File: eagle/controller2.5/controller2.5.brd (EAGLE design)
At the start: 55.9 x 44.5 mm, 42 parts, among them U1 ATMEGA328P, X1 1501_04

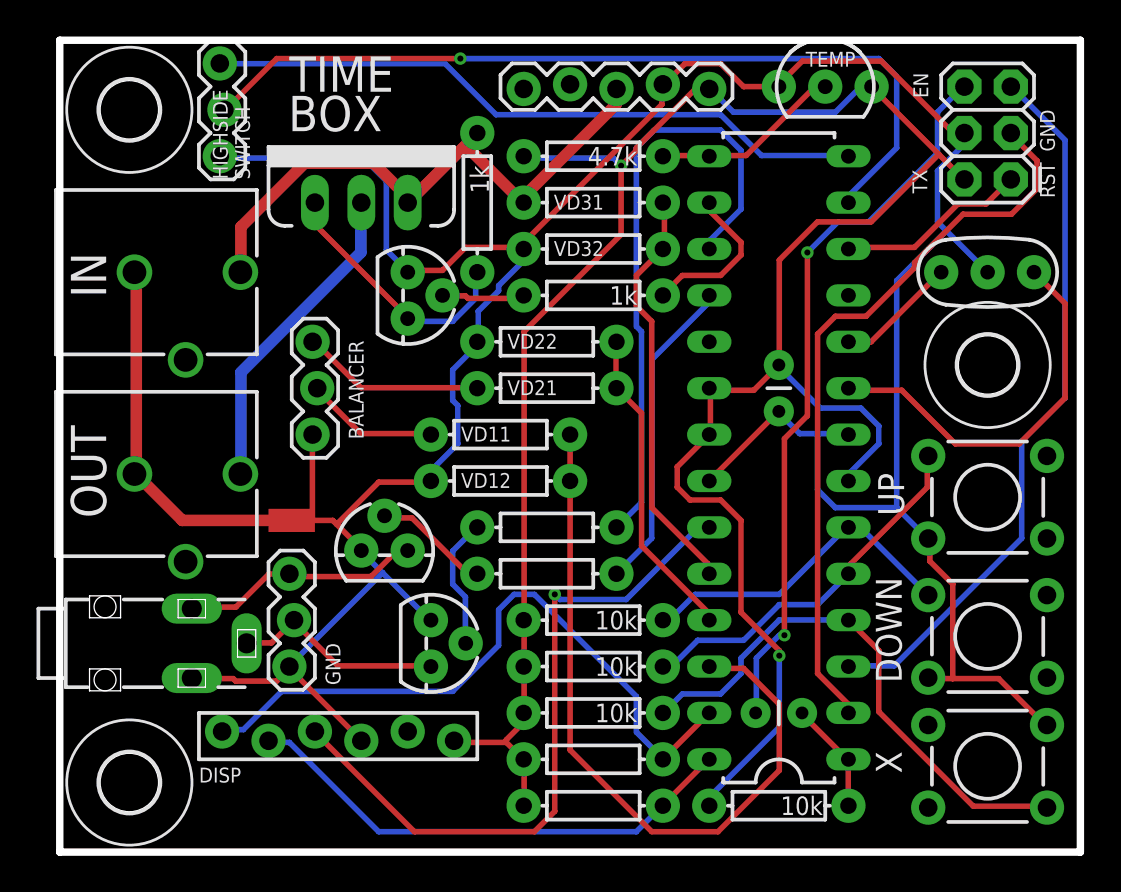
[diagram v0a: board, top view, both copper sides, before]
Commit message: controller2.5: production version
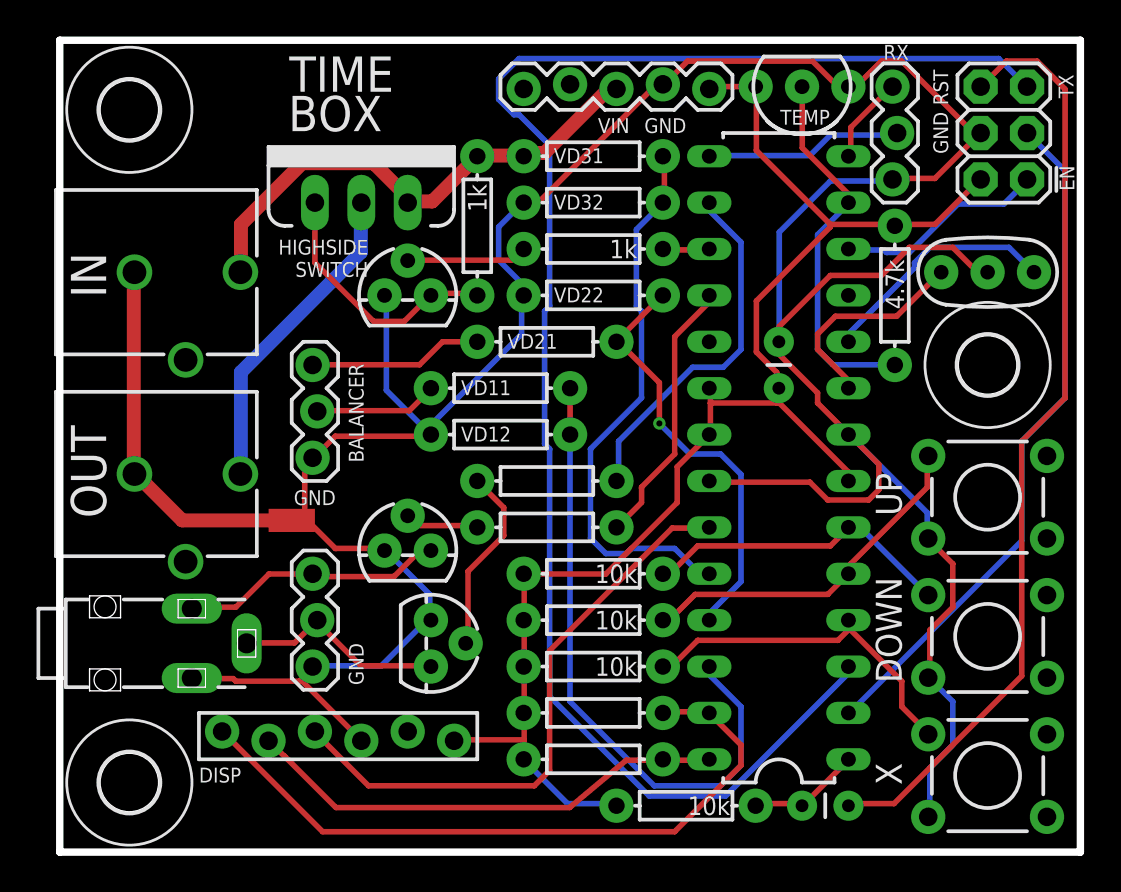
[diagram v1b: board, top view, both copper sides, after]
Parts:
- moved SOFT_SERIAL 36.9 mm to (45.7, 36.8)
- moved RTEMP 18.2 mm to (45.7, 30.5), turned to 90 degrees
- moved C1 7.18 mm to (43.2, 2.54), turned to 180 degrees
- moved R3 5.08 mm to (34.3, 2.54)
- moved C3 3.81 mm to (39.4, 27.9), turned to 270 degrees
- moved VD22 3.59 mm to (29.2, 30.5)
- moved R10 2.54 mm to (29.2, 33.0)
- moved VD21 2.54 mm to (26.7, 27.9)
- moved R7 2.54 mm to (26.7, 17.8)
- moved RB1 2.54 mm to (29.2, 15.2)
- moved R1 2.54 mm to (29.2, 7.62)
- moved R2 2.54 mm to (29.2, 5.08)
- moved RB3 2.54 mm to (29.2, 10.2)
- moved R6 2.54 mm to (26.7, 20.3)
- moved RB2 2.54 mm to (29.2, 12.7)
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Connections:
- removed net DISP_EN: U1.11
- removed net FOO2: U1.19
- net CAM2: now also U1.16; no longer U1.17
- net CAM_EN: now also U1.17; no longer U1.16
- net SOFT_TX: now also U1.15; no longer U1.13
- net TEMP: now also U1.13; no longer U1.15
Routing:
- net VCC: track 130.9 -> 80.8 mm, vias 2 -> 0
- net TX: track 39.3 -> 87.2 mm
- net SOFT_TX: track 46.4 -> 10.9 mm, vias 1 -> 0
- net SOFT_RX: track 36.5 -> 4.88 mm
- net CAM2: track 34.2 -> 19.8 mm
- net RST: track 40.2 -> 51.4 mm, vias 2 -> 0
- net BTN3: track 29.8 -> 19.6 mm
- net TEMP: track 10.5 -> 20.7 mm
- net N$9: track 21.7 -> 11.8 mm
- net VD_DIRECT: track 22.6 -> 30.4 mm
- net N$8: track 6.65 -> 13.4 mm
- net CAM_EN: track 8.79 -> 2.57 mm
- net CELL2: track 17.4 -> 23.5 mm, vias 0 -> 1
- net GND: track 169.9 -> 175.4 mm
- net DISP_RST: track 38.0 -> 32.5 mm, vias 1 -> 0
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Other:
- board text added: "RX"
- board text added: "VIN"
